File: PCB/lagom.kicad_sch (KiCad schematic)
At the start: 167 parts, among them J1 Conn_01x04, J2 Conn_01x03, SW83 RotaryEncoder_Switch, SW84 RotaryEncoder_Switch, U1 ProMicro, U2 74HC138, U3 74HC138

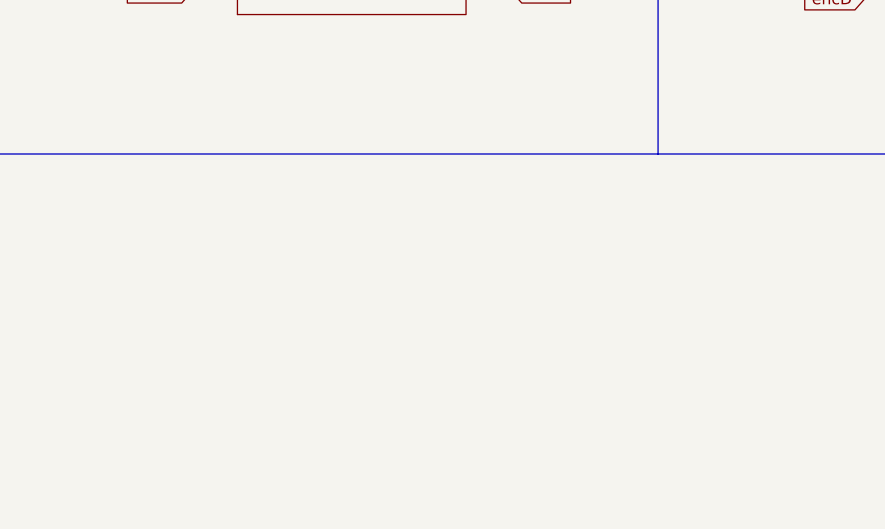
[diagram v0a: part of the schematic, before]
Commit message: Working firmware and updated build guide
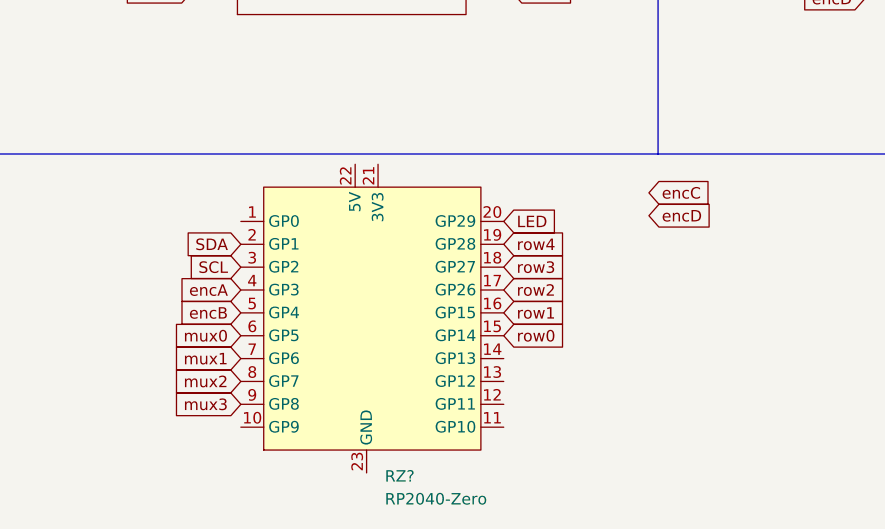
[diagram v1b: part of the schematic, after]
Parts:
- added RZ?: RP2040-Zero, symbol rp2040-zero:RP2040-Zero
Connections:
- net LED: now also RZ?.20 (GP29)
- net SCL: now also RZ?.3 (GP2)
- net SDA: now also RZ?.2 (GP1)
- net encA: now also RZ?.4 (GP3)
- net encB: now also RZ?.5 (GP4)
- net mux0: now also RZ?.6 (GP5)
- net mux1: now also RZ?.7 (GP6)
- net mux2: now also RZ?.8 (GP7)
- net mux3: now also RZ?.9 (GP8)
- net row0: now also RZ?.15 (GP14)
- net row1: now also RZ?.16 (GP15)
- net row2: now also RZ?.17 (GP26)
- net row3: now also RZ?.18 (GP27)
- net row4: now also RZ?.19 (GP28)
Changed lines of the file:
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@@
     (effects (font (size 1.27 1.27)) (justify left bottom))
   )
+  (global_label "encD" (shape input) (at 107.569 223.774 0) (fields_autoplaced)
+    (effects (font (size 1.27 1.27)) (justify left))
+    (property "Intersheet References" "${INTERSHEET_REFS}" (id 0) (at 114.5783 223.6946 0)
+      (effects (font (size 1.27 1.27)) (justify left) hide)
+    )
+  )
   (global_label "col6" (shape input) (at 197.104 40.132 90) (fields_autoplaced)
     (effects (font (size 1.27 1.27)) (justify left))
@@
     )
   )
+  (global_label "LED" (shape input) (at 91.44 224.409 0) (fields_autoplaced)
+    (effects (font (size 1.27 1.27)) (justify left))
+    (property "Intersheet References" "${INTERSHEET_REFS}" (id 0) (at 97.3002 224.4884 0)
+      (effects (font (size 1.27 1.27)) (justify left) hide)
+    )
+  )
   (global_label "LED" (shape input) (at 92.329 186.182 0) (fields_autoplaced)
     (effects (font (size 1.27 1.27)) (justify left))
@@
     )
   )
+  (global_label "row4" (shape input) (at 91.44 226.949 0) (fields_autoplaced)
+    (effects (font (size 1.27 1.27)) (justify left))
+    (property "Intersheet References" "${INTERSHEET_REFS}" (id 0) (at 98.3283 227.0284 0)
+      (effects (font (size 1.27 1.27)) (justify left) hide)
+    )
+  )
   (global_label "RotC" (shape input) (at 373.126 88.773 0) (fields_autoplaced)
     (effects (font (size 1.27 1.27)) (justify left))
@@
     )
   )
+  (global_label "row1" (shape input) (at 91.44 234.569 0) (fields_autoplaced)
+    (effects (font (size 1.27 1.27)) (justify left))
+    (property "Intersheet References" "${INTERSHEET_REFS}" (id 0) (at 98.3283 234.6484 0)
+      (effects (font (size 1.27 1.27)) (justify left) hide)
+    )
+  )
   (global_label "col2" (shape input) (at 297.18 177.673 0) (fields_autoplaced)
     (effects (font (size 1.27 1.27)) (justify left))
@@
     )
   )
+  (global_label "mux0" (shape input) (at 62.23 237.109 180) (fields_autoplaced)
+    (effects (font (size 1.27 1.27)) (justify right))
+    (property "Intersheet References" "${INTERSHEET_REFS}" (id 0) (at 54.7369 237.1884 0)
+      (effects (font (size 1.27 1.27)) (justify right) hide)
+    )
+  )
   (global_label "col13" (shape input) (at 356.489 184.912 0) (fields_autoplaced)
     (effects (font (size 1.27 1.27)) (justify left))
@@
     )
   )
+  (global_label "mux1" (shape input) (at 62.23 239.649 180) (fields_autoplaced)
+    (effects (font (size 1.27 1.27)) (justify right))
+    (property "Intersheet References" "${INTERSHEET_REFS}" (id 0) (at 54.7369 239.7284 0)
+      (effects (font (size 1.27 1.27)) (justify right) hide)
+    )
+  )
   (global_label "mux3" (shape input) (at 338.709 184.912 180) (fields_autoplaced)
     (effects (font (size 1.27 1.27)) (justify right))
@@
     )
   )
+  (global_label "encC" (shape input) (at 107.569 221.234 0) (fields_autoplaced)
+    (effects (font (size 1.27 1.27)) (justify left))
+    (property "Intersheet References" "${INTERSHEET_REFS}" (id 0) (at 114.5783 221.1546 0)
+      (effects (font (size 1.27 1.27)) (justify left) hide)
+    )
+  )
+  (global_label "row3" (shape input) (at 91.44 229.489 0) (fields_autoplaced)
+    (effects (font (size 1.27 1.27)) (justify left))
+    (property "Intersheet References" "${INTERSHEET_REFS}" (id 0) (at 98.3283 229.5684 0)
+      (effects (font (size 1.27 1.27)) (justify left) hide)
+    )
+  )
+  (global_label "encB" (shape input) (at 62.23 234.569 180) (fields_autoplaced)
+    (effects (font (size 1.27 1.27)) (justify right))
+    (property "Intersheet References" "${INTERSHEET_REFS}" (id 0) (at 55.2207 234.6484 0)
+      (effects (font (size 1.27 1.27)) (justify right) hide)
+    )
+  )
   (global_label "col12" (shape input) (at 326.136 40.005 90) (fields_autoplaced)
     (effects (font (size 1.27 1.27)) (justify left))
@@
     )
   )
+  (global_label "SDA" (shape input) (at 62.23 226.949 180) (fields_autoplaced)
+    (effects (font (size 1.27 1.27)) (justify right))
+    (property "Intersheet References" "${INTERSHEET_REFS}" (id 0) (at 56.2488 226.8696 0)
+      (effects (font (size 1.27 1.27)) (justify right) hide)
+    )
+  )
   (global_label "row1" (shape input) (at 49.784 74.549 180) (fields_autoplaced)
     (effects (font (size 1.27 1.27)) (justify right))
@@
     )
   )
+  (global_label "row2" (shape input) (at 91.44 232.029 0) (fields_autoplaced)
+    (effects (font (size 1.27 1.27)) (justify left))
+    (property "Intersheet References" "${INTERSHEET_REFS}" (id 0) (at 98.3283 232.1084 0)
+      (effects (font (size 1.27 1.27)) (justify left) hide)
+    )
+  )
   (global_label "row3" (shape input) (at 92.329 191.262 0) (fields_autoplaced)
     (effects (font (size 1.27 1.27)) (justify left))
@@
     )
   )
+  (global_label "SCL" (shape input) (at 62.23 229.489 180) (fields_autoplaced)
+    (effects (font (size 1.27 1.27)) (justify right))
+    (property "Intersheet References" "${INTERSHEET_REFS}" (id 0) (at 56.3093 229.4096 0)
+      (effects (font (size 1.27 1.27)) (justify right) hide)
+    )
+  )
   (global_label "encB" (shape input) (at 56.769 188.722 180) (fields_autoplaced)
     (effects (font (size 1.27 1.27)) (justify right))
@@
     )
   )
+  (global_label "mux2" (shape input) (at 62.23 242.189 180) (fields_autoplaced)
+    (effects (font (size 1.27 1.27)) (justify right))
+    (property "Intersheet References" "${INTERSHEET_REFS}" (id 0) (at 54.7369 242.2684 0)
+      (effects (font (size 1.27 1.27)) (justify right) hide)
+    )
+  )
+  (global_label "encA" (shape input) (at 62.23 232.029 180) (fields_autoplaced)
+    (effects (font (size 1.27 1.27)) (justify right))
+    (property "Intersheet References" "${INTERSHEET_REFS}" (id 0) (at 55.4021 232.1084 0)
+      (effects (font (size 1.27 1.27)) (justify right) hide)
+    )
+  )
   (global_label "col0" (shape input) (at 297.18 172.593 0) (fields_autoplaced)
     (effects (font (size 1.27 1.27)) (justify left))
@@
     )
   )
+  (global_label "row0" (shape input) (at 91.44 237.109 0) (fields_autoplaced)
+    (effects (font (size 1.27 1.27)) (justify left))
+    (property "Intersheet References" "${INTERSHEET_REFS}" (id 0) (at 98.3283 237.1884 0)
+      (effects (font (size 1.27 1.27)) (justify left) hide)
+    )
+  )
   (global_label "col6" (shape input) (at 297.18 187.833 0) (fields_autoplaced)
     (effects (font (size 1.27 1.27)) (justify left))
@@
     )
   )
+  (global_label "mux3" (shape input) (at 62.23 244.729 180) (fields_autoplaced)
+    (effects (font (size 1.27 1.27)) (justify right))
+    (property "Intersheet References" "${INTERSHEET_REFS}" (id 0) (at 54.7369 244.8084 0)
+      (effects (font (size 1.27 1.27)) (justify right) hide)
+    )
+  )
   (symbol (lib_id "keyboard_parts:KEYSW") (at 232.029 88.773 0) (unit 1)
     (in_bom yes) (on_board yes)
@@
     (pin "1")
   )
+  (symbol (lib_id "rp2040-zero:RP2040-Zero") (at 76.2 234.569 0) (unit 1)
+    (in_bom yes) (on_board yes) (fields_autoplaced)
+    (property "Reference" "RZ?" (id 0) (at 78.2194 252.73 0)
+      (effects (font (size 1.27 1.27)) (justify left))
+    )
+    (property "Value" "RP2040-Zero" (id 1) (at 78.2194 255.27 0)
+      (effects (font (size 1.27 1.27)) (justify left))
+    )
+    (property "Footprint" "" (id 2) (at 76.2 234.569 0)
+      (effects (font (size 1.27 1.27)) hide)
+    )
+    (property "Datasheet" "" (id 3) (at 76.2 234.569 0)
+      (effects (font (size 1.27 1.27)) hide)
+    )
+    (pin "1")
+    (pin "10")
+    (pin "11")
+    (pin "12")
+    (pin "13")
+    (pin "14")
+    (pin "15")
+    (pin "16")
+    (pin "17")
+    (pin "18")
+    (pin "19")
+    (pin "2")
+    (pin "20")
+    (pin "21")
+    (pin "22")
+    (pin "23")
+    (pin "3")
+    (pin "4")
+    (pin "5")
+    (pin "6")
+    (pin "7")
+    (pin "8")
+    (pin "9")
+  )
   (symbol (lib_id "keyboard_parts:KEYSW") (at 189.484 68.199 0) (unit 1)
     (in_bom yes) (on_board yes)
@@
       (reference "J2") (unit 1) (value "Conn_01x03") (footprint "Connector_PinSocket_2.54mm:PinSocket_1x03_P2.54mm_Vertical")
     )
+    (path "/2b8cd22b-41b0-4a3f-b88d-8b74deac8136"
+      (reference "RZ?") (unit 1) (value "RP2040-Zero") (footprint "")
+    )
     (path "/7d924492-06b9-4e8b-ad72-2209ecf70752"

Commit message: Build guide updated to show LED socket
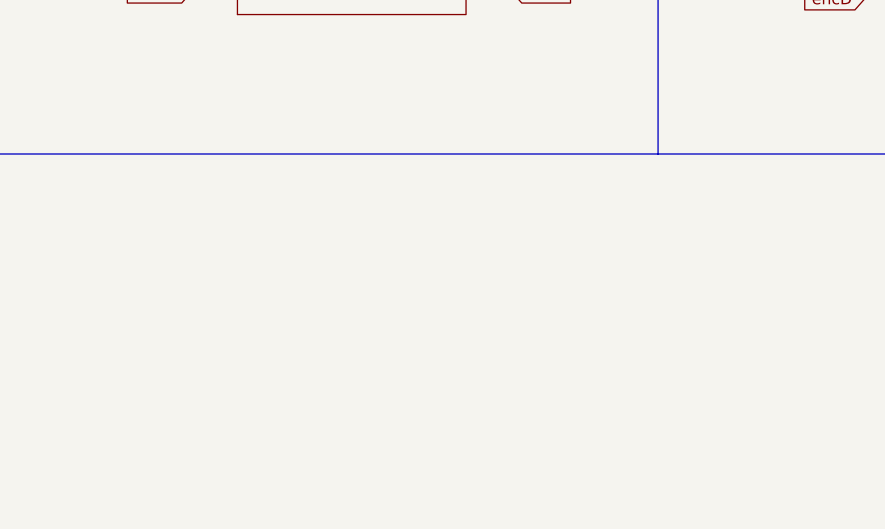
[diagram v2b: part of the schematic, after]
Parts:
- removed RZ?: RP2040-Zero, symbol rp2040-zero:RP2040-Zero
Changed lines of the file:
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@@
     (effects (font (size 1.27 1.27)) (justify left bottom))
   )
-  (global_label "encD" (shape input) (at 107.569 223.774 0) (fields_autoplaced)
-    (effects (font (size 1.27 1.27)) (justify left))
-    (property "Intersheet References" "${INTERSHEET_REFS}" (id 0) (at 114.5783 223.6946 0)
-      (effects (font (size 1.27 1.27)) (justify left) hide)
-    )
-  )
   (global_label "col6" (shape input) (at 197.104 40.132 90) (fields_autoplaced)
     (effects (font (size 1.27 1.27)) (justify left))
@@
     )
   )
-  (global_label "LED" (shape input) (at 91.44 224.409 0) (fields_autoplaced)
-    (effects (font (size 1.27 1.27)) (justify left))
-    (property "Intersheet References" "${INTERSHEET_REFS}" (id 0) (at 97.3002 224.4884 0)
-      (effects (font (size 1.27 1.27)) (justify left) hide)
-    )
-  )
   (global_label "LED" (shape input) (at 92.329 186.182 0) (fields_autoplaced)
     (effects (font (size 1.27 1.27)) (justify left))
@@
     )
   )
-  (global_label "row4" (shape input) (at 91.44 226.949 0) (fields_autoplaced)
-    (effects (font (size 1.27 1.27)) (justify left))
-    (property "Intersheet References" "${INTERSHEET_REFS}" (id 0) (at 98.3283 227.0284 0)
-      (effects (font (size 1.27 1.27)) (justify left) hide)
-    )
-  )
   (global_label "RotC" (shape input) (at 373.126 88.773 0) (fields_autoplaced)
     (effects (font (size 1.27 1.27)) (justify left))
@@
     )
   )
-  (global_label "row1" (shape input) (at 91.44 234.569 0) (fields_autoplaced)
-    (effects (font (size 1.27 1.27)) (justify left))
-    (property "Intersheet References" "${INTERSHEET_REFS}" (id 0) (at 98.3283 234.6484 0)
-      (effects (font (size 1.27 1.27)) (justify left) hide)
-    )
-  )
   (global_label "col2" (shape input) (at 297.18 177.673 0) (fields_autoplaced)
     (effects (font (size 1.27 1.27)) (justify left))
@@
     )
   )
-  (global_label "mux0" (shape input) (at 62.23 237.109 180) (fields_autoplaced)
-    (effects (font (size 1.27 1.27)) (justify right))
-    (property "Intersheet References" "${INTERSHEET_REFS}" (id 0) (at 54.7369 237.1884 0)
-      (effects (font (size 1.27 1.27)) (justify right) hide)
-    )
-  )
   (global_label "col13" (shape input) (at 356.489 184.912 0) (fields_autoplaced)
     (effects (font (size 1.27 1.27)) (justify left))
@@
     )
   )
-  (global_label "mux1" (shape input) (at 62.23 239.649 180) (fields_autoplaced)
-    (effects (font (size 1.27 1.27)) (justify right))
-    (property "Intersheet References" "${INTERSHEET_REFS}" (id 0) (at 54.7369 239.7284 0)
-      (effects (font (size 1.27 1.27)) (justify right) hide)
-    )
-  )
   (global_label "mux3" (shape input) (at 338.709 184.912 180) (fields_autoplaced)
     (effects (font (size 1.27 1.27)) (justify right))
@@
     )
   )
-  (global_label "encC" (shape input) (at 107.569 221.234 0) (fields_autoplaced)
-    (effects (font (size 1.27 1.27)) (justify left))
-    (property "Intersheet References" "${INTERSHEET_REFS}" (id 0) (at 114.5783 221.1546 0)
-      (effects (font (size 1.27 1.27)) (justify left) hide)
-    )
-  )
-  (global_label "row3" (shape input) (at 91.44 229.489 0) (fields_autoplaced)
-    (effects (font (size 1.27 1.27)) (justify left))
-    (property "Intersheet References" "${INTERSHEET_REFS}" (id 0) (at 98.3283 229.5684 0)
-      (effects (font (size 1.27 1.27)) (justify left) hide)
-    )
-  )
-  (global_label "encB" (shape input) (at 62.23 234.569 180) (fields_autoplaced)
-    (effects (font (size 1.27 1.27)) (justify right))
-    (property "Intersheet References" "${INTERSHEET_REFS}" (id 0) (at 55.2207 234.6484 0)
-      (effects (font (size 1.27 1.27)) (justify right) hide)
-    )
-  )
   (global_label "col12" (shape input) (at 326.136 40.005 90) (fields_autoplaced)
     (effects (font (size 1.27 1.27)) (justify left))
@@
     )
   )
-  (global_label "SDA" (shape input) (at 62.23 226.949 180) (fields_autoplaced)
-    (effects (font (size 1.27 1.27)) (justify right))
-    (property "Intersheet References" "${INTERSHEET_REFS}" (id 0) (at 56.2488 226.8696 0)
-      (effects (font (size 1.27 1.27)) (justify right) hide)
-    )
-  )
   (global_label "row1" (shape input) (at 49.784 74.549 180) (fields_autoplaced)
     (effects (font (size 1.27 1.27)) (justify right))
@@
     )
   )
-  (global_label "row2" (shape input) (at 91.44 232.029 0) (fields_autoplaced)
-    (effects (font (size 1.27 1.27)) (justify left))
-    (property "Intersheet References" "${INTERSHEET_REFS}" (id 0) (at 98.3283 232.1084 0)
-      (effects (font (size 1.27 1.27)) (justify left) hide)
-    )
-  )
   (global_label "row3" (shape input) (at 92.329 191.262 0) (fields_autoplaced)
     (effects (font (size 1.27 1.27)) (justify left))
@@
     )
   )
-  (global_label "SCL" (shape input) (at 62.23 229.489 180) (fields_autoplaced)
-    (effects (font (size 1.27 1.27)) (justify right))
-    (property "Intersheet References" "${INTERSHEET_REFS}" (id 0) (at 56.3093 229.4096 0)
-      (effects (font (size 1.27 1.27)) (justify right) hide)
-    )
-  )
   (global_label "encB" (shape input) (at 56.769 188.722 180) (fields_autoplaced)
     (effects (font (size 1.27 1.27)) (justify right))
@@
     )
   )
-  (global_label "mux2" (shape input) (at 62.23 242.189 180) (fields_autoplaced)
-    (effects (font (size 1.27 1.27)) (justify right))
-    (property "Intersheet References" "${INTERSHEET_REFS}" (id 0) (at 54.7369 242.2684 0)
-      (effects (font (size 1.27 1.27)) (justify right) hide)
-    )
-  )
-  (global_label "encA" (shape input) (at 62.23 232.029 180) (fields_autoplaced)
-    (effects (font (size 1.27 1.27)) (justify right))
-    (property "Intersheet References" "${INTERSHEET_REFS}" (id 0) (at 55.4021 232.1084 0)
-      (effects (font (size 1.27 1.27)) (justify right) hide)
-    )
-  )
   (global_label "col0" (shape input) (at 297.18 172.593 0) (fields_autoplaced)
     (effects (font (size 1.27 1.27)) (justify left))
@@
     )
   )
-  (global_label "row0" (shape input) (at 91.44 237.109 0) (fields_autoplaced)
-    (effects (font (size 1.27 1.27)) (justify left))
-    (property "Intersheet References" "${INTERSHEET_REFS}" (id 0) (at 98.3283 237.1884 0)
-      (effects (font (size 1.27 1.27)) (justify left) hide)
-    )
-  )
   (global_label "col6" (shape input) (at 297.18 187.833 0) (fields_autoplaced)
     (effects (font (size 1.27 1.27)) (justify left))
@@
     )
   )
-  (global_label "mux3" (shape input) (at 62.23 244.729 180) (fields_autoplaced)
-    (effects (font (size 1.27 1.27)) (justify right))
-    (property "Intersheet References" "${INTERSHEET_REFS}" (id 0) (at 54.7369 244.8084 0)
-      (effects (font (size 1.27 1.27)) (justify right) hide)
-    )
-  )
   (symbol (lib_id "keyboard_parts:KEYSW") (at 232.029 88.773 0) (unit 1)
     (in_bom yes) (on_board yes)
@@
     (pin "1")
   )
-  (symbol (lib_id "rp2040-zero:RP2040-Zero") (at 76.2 234.569 0) (unit 1)
-    (in_bom yes) (on_board yes) (fields_autoplaced)
-    (property "Reference" "RZ?" (id 0) (at 78.2194 252.73 0)
-      (effects (font (size 1.27 1.27)) (justify left))
-    )
-    (property "Value" "RP2040-Zero" (id 1) (at 78.2194 255.27 0)
-      (effects (font (size 1.27 1.27)) (justify left))
-    )
-    (property "Footprint" "" (id 2) (at 76.2 234.569 0)
-      (effects (font (size 1.27 1.27)) hide)
-    )
-    (property "Datasheet" "" (id 3) (at 76.2 234.569 0)
-      (effects (font (size 1.27 1.27)) hide)
-    )
-    (pin "1")
-    (pin "10")
-    (pin "11")
-    (pin "12")
-    (pin "13")
-    (pin "14")
-    (pin "15")
-    (pin "16")
-    (pin "17")
-    (pin "18")
-    (pin "19")
-    (pin "2")
-    (pin "20")
-    (pin "21")
-    (pin "22")
-    (pin "23")
-    (pin "3")
-    (pin "4")
-    (pin "5")
-    (pin "6")
-    (pin "7")
-    (pin "8")
-    (pin "9")
-  )
   (symbol (lib_id "keyboard_parts:KEYSW") (at 189.484 68.199 0) (unit 1)
     (in_bom yes) (on_board yes)
@@
       (reference "J2") (unit 1) (value "Conn_01x03") (footprint "Connector_PinSocket_2.54mm:PinSocket_1x03_P2.54mm_Vertical")
     )
-    (path "/2b8cd22b-41b0-4a3f-b88d-8b74deac8136"
-      (reference "RZ?") (unit 1) (value "RP2040-Zero") (footprint "")
-    )
     (path "/7d924492-06b9-4e8b-ad72-2209ecf70752"
